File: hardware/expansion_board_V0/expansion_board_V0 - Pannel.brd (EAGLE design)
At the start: 212 x 132 mm, 555 parts, among them CON1 ELEC, CON10 M5, CON11 M2, CON12 M4, CON13 M1, CON14 ESC0, CON15 CON10_2_2.54, CON16 CON10_2_2.54, CON17 ESC1, CON18 UART0, CON19 QEI1, CON2 SERVO, CON20 AN0, CON21 S0, CON22 IO0, CON23 AN1, CON24 S1, CON25 IO1, CON26 UART1, CON27 QEI0, CON28 AN2, CON29 S2, CON3 LIPO_MOT, CON30 IO2, CON31 TELEM, CON32 QEI3, CON33 AN3, CON34 S3, CON35 IO3, CON36 BALISE, CON37 AN4, CON38 S4, CON39 IO4, CON4 LIPO_MOT, CON40 SPI0, CON41 QEI2, CON42 AN5, CON43 S5, CON44 IO5, CON45 SPI1, CON46 AN6, CON47 S6, CON48 IO6, CON49 I2C0, CON5 LIPO_MOT, CON50 AN7, CON51 S7, CON52 IO7, CON53 I2C1, CON54 USB2, CON55 USB3, CON56 USBfpga, CON57 FPGA_GPIO0, CON58 FPGA_GPIO1, CON59 FPGA_LTC, CON6 LIPO_MOT, CON60 USB3, CON61 CON5_2.54S, CON62 CON5_2.54S, CON63 CON5_2.54S, CON64 CON5_2.54S, CON65 CON5_2.54S, CON66 CON5_2.54S, CON67 CON5_2.54S, CON68 CON5_2.54S, CON69 CON5_2.54S, CON7 FPGApower, CON70 CON5_2.54S, CON71 CON5_2.54S, CON72 CON5_2.54S, CON73 CON5_2.54S, CON74 CON5_2.54S, CON75 CON5_2.54S, CON76 CON5_2.54S, CON8 M0, CON9 M3, IC1 ADS1258, IC2 ADS1278, IC3 REF5030I, IC4 REF5025I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

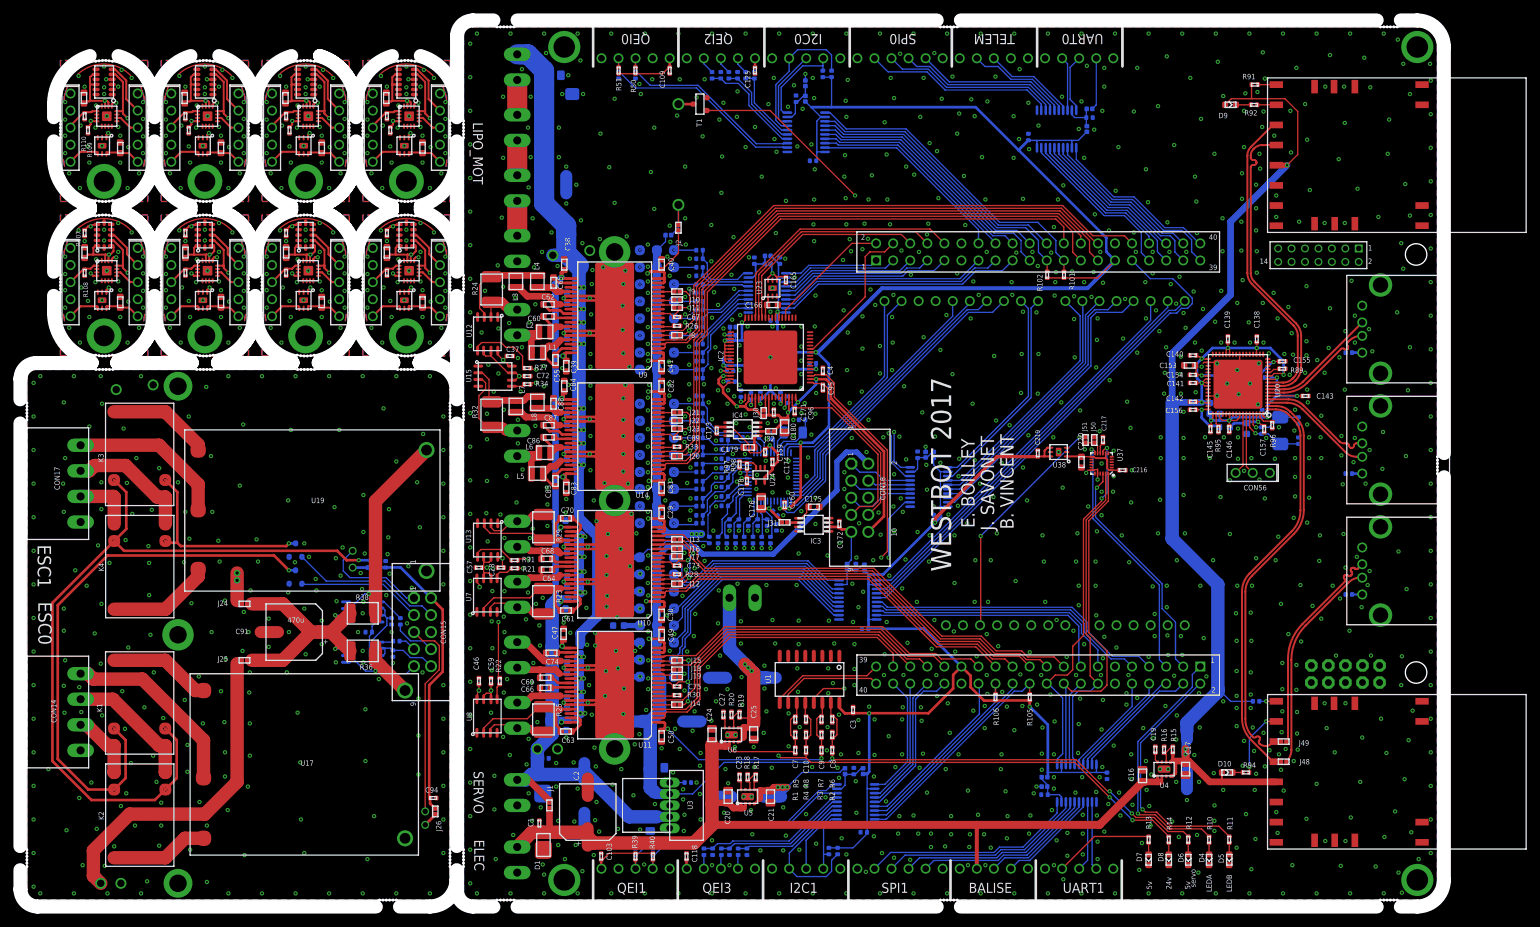
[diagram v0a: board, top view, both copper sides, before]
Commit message: IMU footprint ok Elec posté sur Eurocircuit
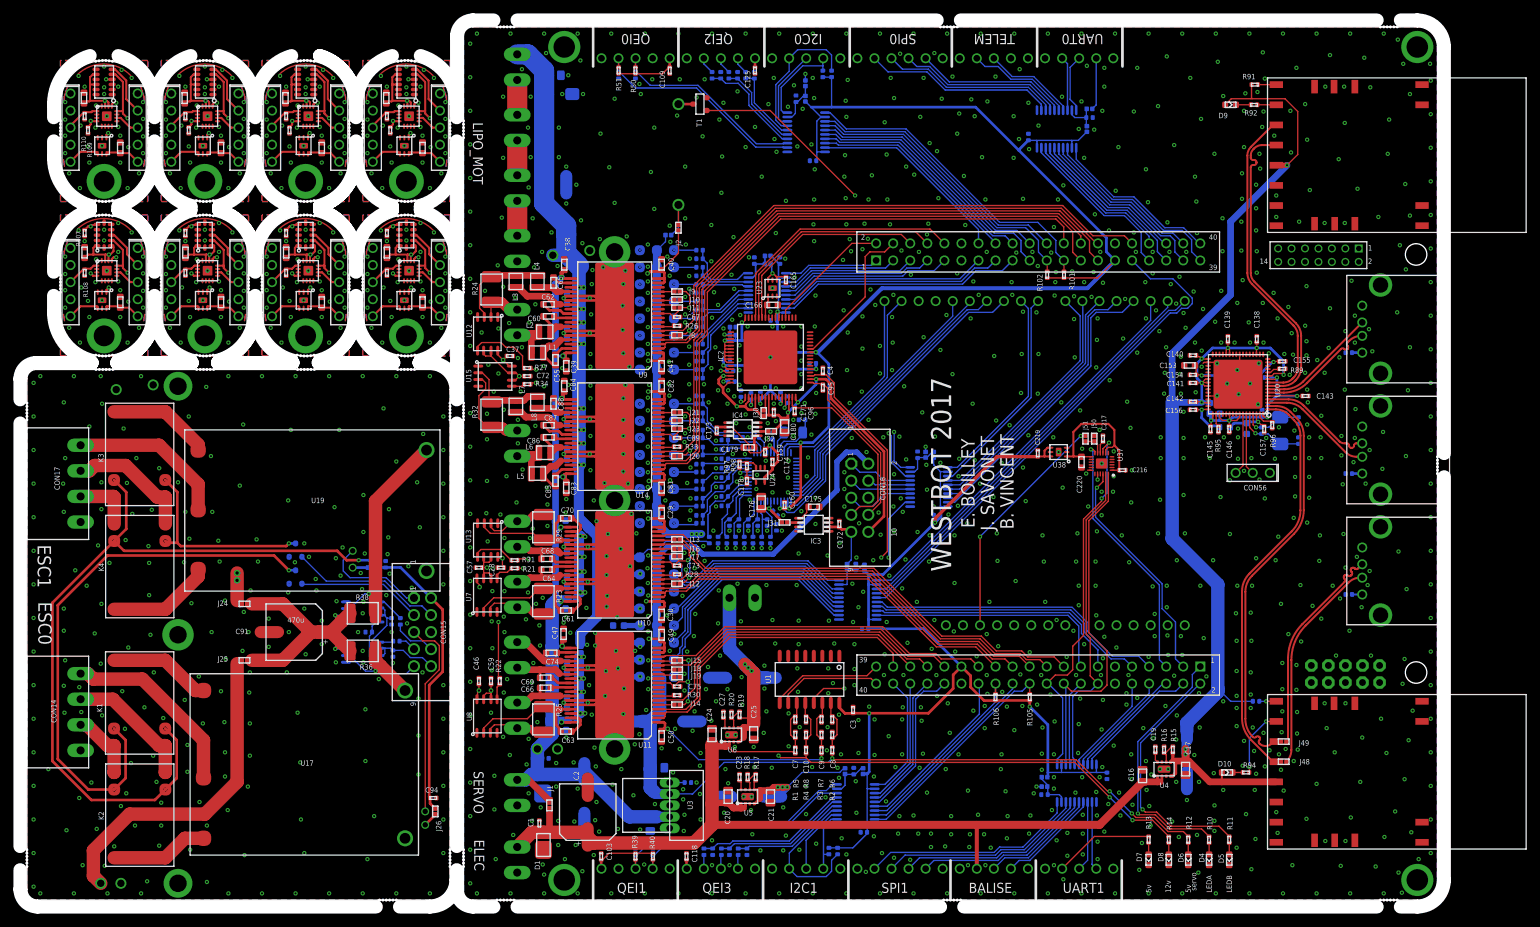
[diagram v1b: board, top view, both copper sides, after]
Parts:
- J50, J51: value (none) -> 0
- moved C217 0.20 mm to (-49.8, 3.70)
- moved J50 0.20 mm to (-51.1, 3.70), turned to 270 degrees
- moved J51 0.20 mm to (-52.4, 3.70)
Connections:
- removed net S$1: J51.P$2, U29.RESET
- new net N$98: J50.P$2, J51.P$1, U37.11
- net GND: now also J50.P$1, U37.14, U37.15, U37.16, U37.17, U37.2, U37.3, U37.4, U37.5, U37.6, U37.PAD; no longer J50.P$2
- net IMU_FSYNC: now also J51.P$2, U29.RESET; no longer J50.P$1, J51.P$1, U37.11
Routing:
- net S$1: track 35.0 -> 0.00 mm, vias 2 -> 0
- net IMU_FSYNC: track 3.09 -> 35.1 mm, vias 0 -> 2
- net N$74: track 10.1 -> 23.7 mm
- net N$98: track 0.00 -> 3.24 mm
- net GND: track 244.6 -> 242.9 mm, vias 1566 -> 1564
- net MISO1: track 54.5 -> 56.2 mm
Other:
- outline, holes or cut-outs redrawn
- board text removed: "24v"
